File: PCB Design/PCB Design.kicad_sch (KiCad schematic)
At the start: 0 parts

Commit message: intial circuit implementation
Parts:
- added D1, D2, D3: LED, LED_THT:LED_D3.0mm, symbol Device:LED
- added J1: Conn_01x02_Pin, Connector_Wire:SolderWire-1sqmm_1x02_P5.4mm_D1.4mm_OD2.7mm, symbol Connector:Conn_01x02_Pin
- added R1: 35, Resistor_THT:R_Axial_DIN0207_L6.3mm_D2.5mm_P10.16mm_Horizontal, symbol Device:R
- added SW1: SW_SP3T, Button_Switch_THT:SW_DIP_SPSTx02_Piano_10.8x6.64mm_W7.62mm_P2.54mm, symbol Switch:SW_SP3T
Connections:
- new net: J1.1 (Pin_1), R1.1
- new net: R1.2, SW1.3
- new net: D1.1 (K), D2.1 (K), D3.1 (K), J1.2 (Pin_2)
- new net: D2.2 (A), SW1.2
- new net: D3.2 (A), SW1.1
- new net: D1.2 (A), SW1.4

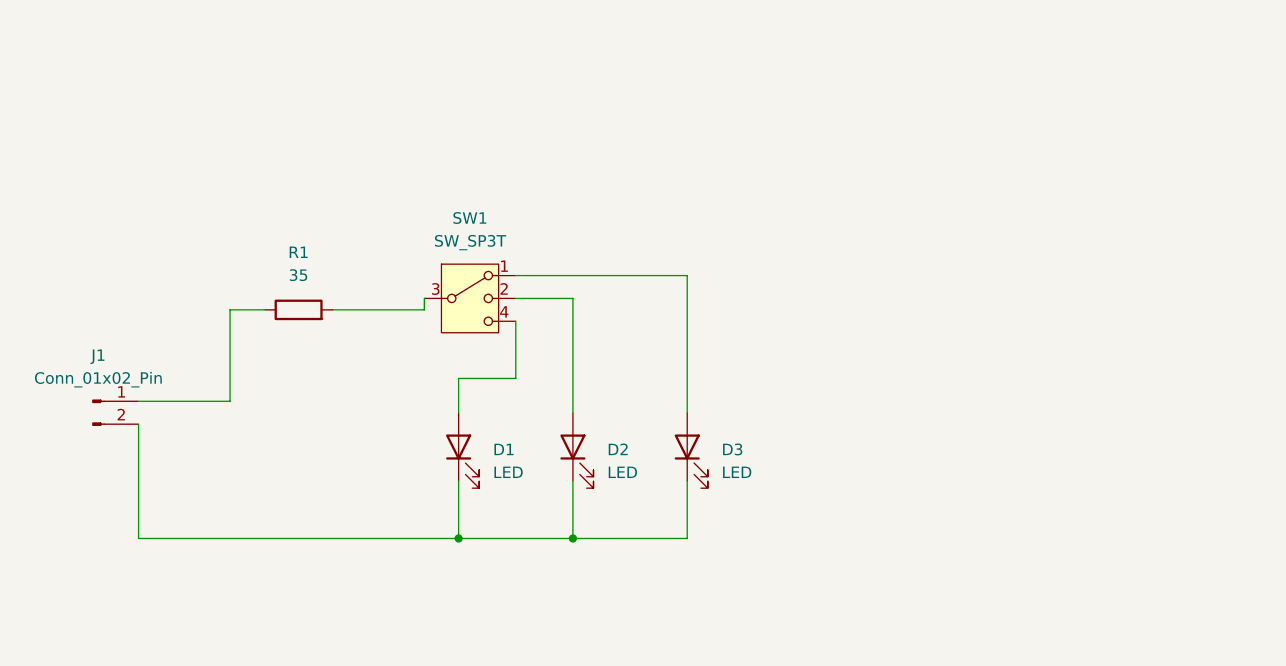
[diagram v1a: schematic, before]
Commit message: adjustements the PCB schematic
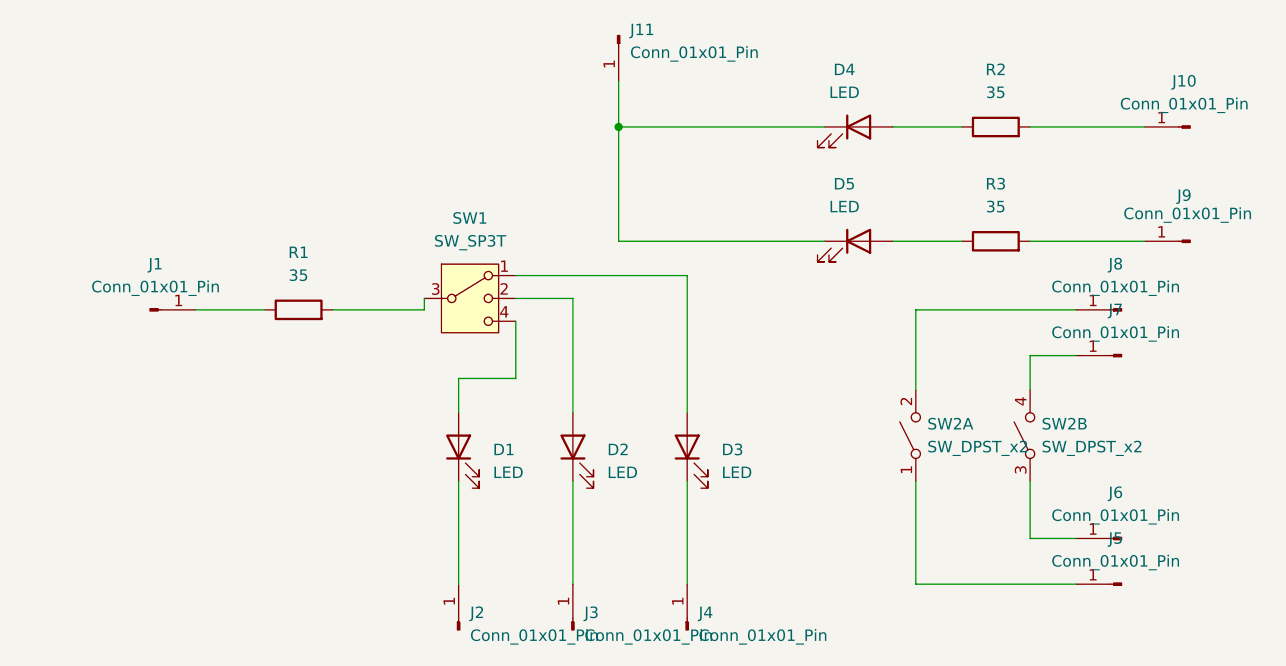
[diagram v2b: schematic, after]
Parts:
- removed J1: Conn_01x02_Pin, Connector_Wire:SolderWire-1sqmm_1x02_P5.4mm_D1.4mm_OD2.7mm, symbol Connector:Conn_01x02_Pin
- added D4, D5: LED, LED_THT:LED_D3.0mm, symbol Device:LED
- added J1, J10, J11, J2, J3, J4, J5, J6, J7, J8, J9: Conn_01x01_Pin, Connector_Wire:SolderWire-1sqmm_1x01_D1.4mm_OD2.7mm, symbol Connector:Conn_01x01_Pin
- added R2, R3: 35, Resistor_THT:R_Axial_DIN0207_L6.3mm_D2.5mm_P10.16mm_Horizontal, symbol Device:R
- added SW2: SW_DPST_x2, symbol Switch:SW_DPST_x2
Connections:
- net at R1.1: now also J1.1 (Pin_1)
- new net: D3.1 (K), J4.1 (Pin_1)
- new net: J9.1 (Pin_1), R3.2
- new net: D2.1 (K), J3.1 (Pin_1)
- new net: J10.1 (Pin_1), R2.2
- new net: J7.1 (Pin_1), SW2.4 (B)
- new net: J8.1 (Pin_1), SW2.2 (B)
- new net: D4.1 (K), D5.1 (K), J11.1 (Pin_1)
- new net: D4.2 (A), R2.1
- new net: D5.2 (A), R3.1
- new net: J5.1 (Pin_1), SW2.1 (A)
- new net: D1.1 (K), J2.1 (Pin_1)
- new net: J6.1 (Pin_1), SW2.3 (A)
